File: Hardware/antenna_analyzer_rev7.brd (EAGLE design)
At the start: 99.1 x 78.7 mm, 42 parts, among them J1 DC_JACK, P1 SOLDER_PAD_35_HOLE, P2 SOLDER_PAD_35_HOLE, P3 SOLDER_PAD_35_HOLE, U1 ARDUINO_PRO_MICRO, U2 AD9850_MOD, U3 6002_OP_AMP, U5 SWITCHING_REGULATOR

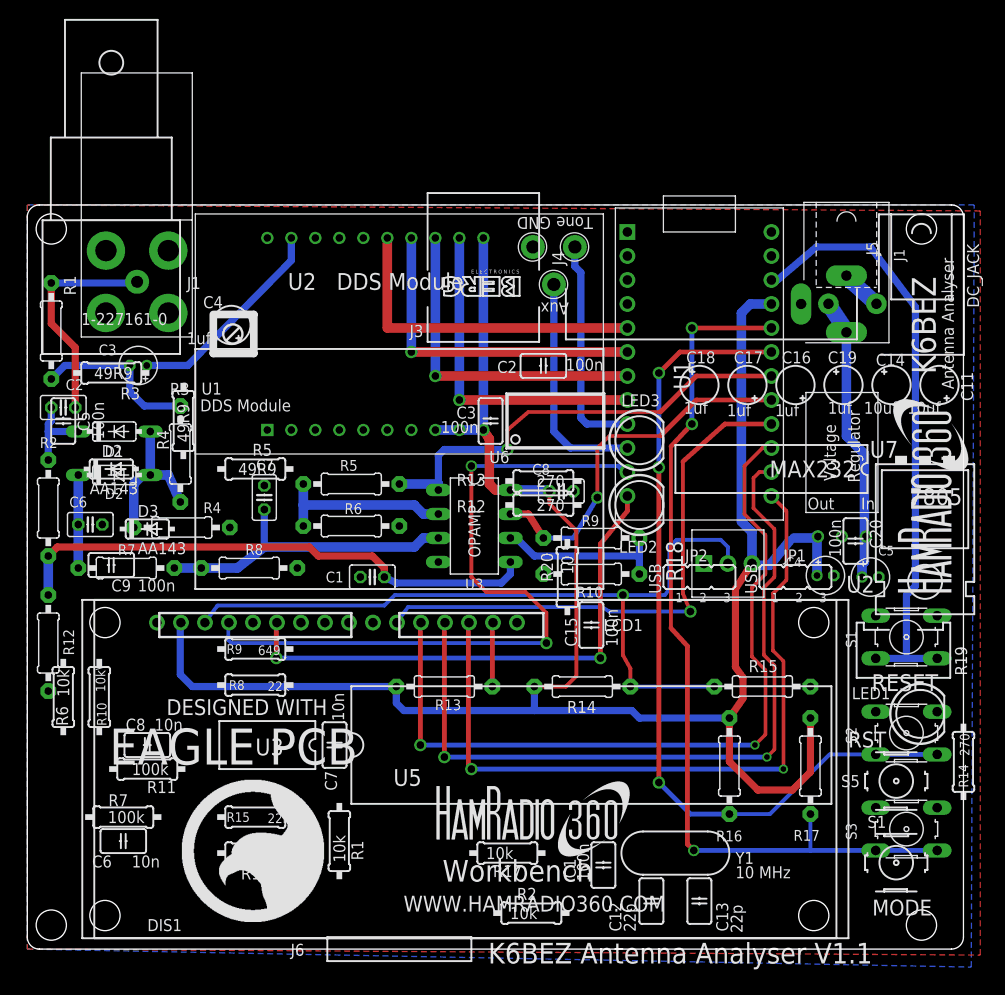
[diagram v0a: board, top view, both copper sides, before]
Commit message: 4X6UB Modifications
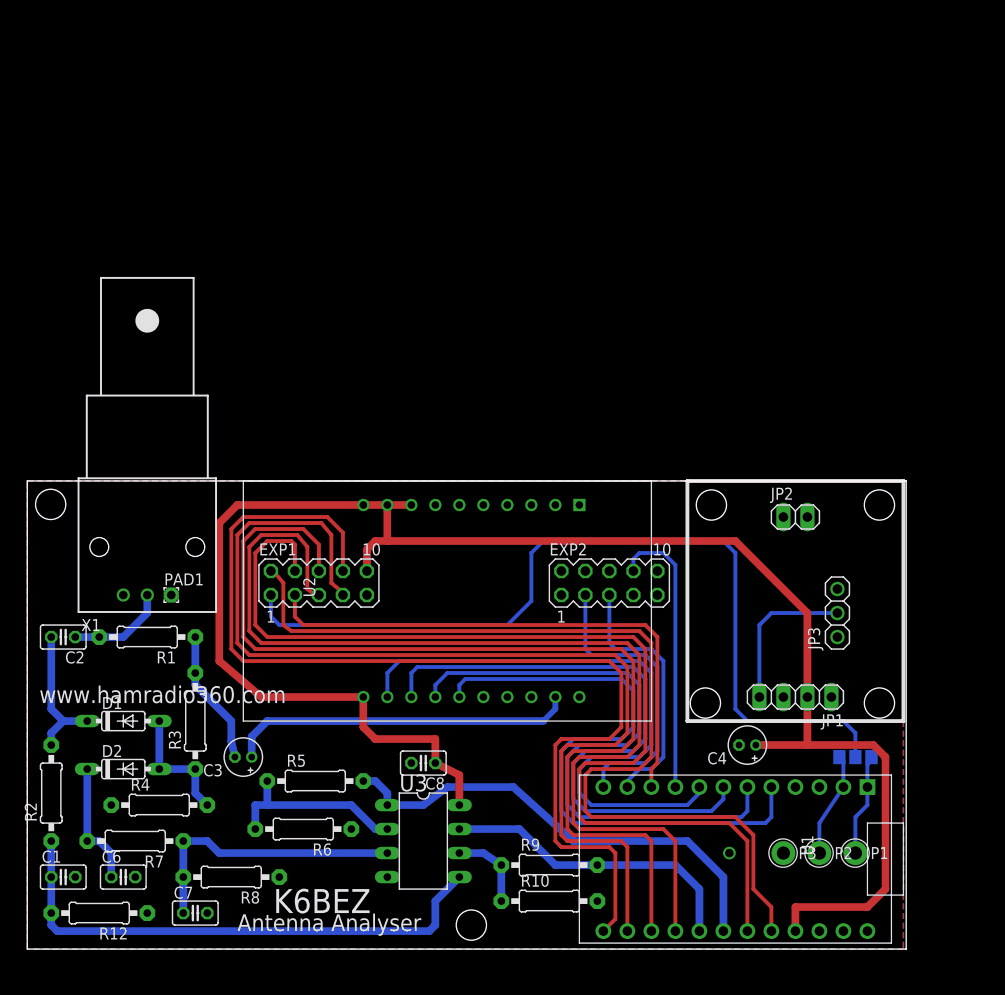
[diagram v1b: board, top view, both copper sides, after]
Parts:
- removed C5: 10uf, resistor:E1,8-4
- removed CON1: (no value), srs_lib_4:BNC-SMALL
- removed J1: DC_JACK, srs_lib_2:DC_COAXIAL_JACK
- removed LCD1: LCD_2_16, srs_lib_4:LCD_2X16
- removed R13: 10, adafruit:0207/10
- removed R14, R16, R17: 10k, adafruit:0207/10
- removed R15: 649, adafruit:0207/10
- removed R18: (no value), Discrete:3362U
- removed S1: RESET, switch-omron:B3F-10XX
- removed S2: MODE, switch-omron:B3F-10XX
- removed S3: BAND, switch-omron:B3F-10XX
- removed U$1, U$2: (no value), Eagle logo:CS-2016-LOGO-15MM
- removed U5: SWITCHING_REGULATOR, srs_new:SWITCHING_REGULATOR
- added EXP1, EXP2: (no value), con-lstb:MA05-2
- added JMP1: 0R-JUMPA, jump-0r-smd:A0R-JMP
- added JP1: (no value), pinhead:1X04
- added JP2: (no value), pinhead:1X02
- added JP3: (no value), adafruit:1X03
- added PAD1: (no value), wirepad:1,6/0,9
- added X1: 1-227161-0, con-coax:AMP_227161
- moved P1 70.7 mm to (87.6, 10.2)
- moved P3 69.4 mm to (80.0, 10.2)
- moved P2 66.4 mm to (83.8, 10.2)
- moved U1 64.0 mm to (88.9, 17.1), turned to 270 degrees
- moved C1 45.6 mm to (3.81, 7.62), turned to 0 degrees
- moved C7 44.6 mm to (17.8, 3.81), turned to 0 degrees
- moved C3 42.9 mm to (22.9, 20.3)
- moved C6 37.5 mm to (10.2, 7.62)
- moved R10 34.9 mm to (55.2, 5.08), turned to 0 degrees
- moved R9 34.9 mm to (55.2, 8.89), turned to 0 degrees
- moved R1 33.9 mm to (12.7, 33.0), turned to 180 degrees
- moved U3 33.8 mm to (41.9, 11.4)
- moved R8 32.8 mm to (21.6, 7.62)
- moved R6 32.5 mm to (29.2, 12.7)
- moved C8 32.3 mm to (41.9, 19.7), turned to 180 degrees
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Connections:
- removed net AUX: P2.1, U1.10
- removed net BAND_SEL: R17.1, S3.3, S3.4, U1.20
- removed net MODE_SEL: R16.1, S2.3, S2.4, U1.19
- removed net N$12: S1.3, S1.4, U1.22
- removed net N$37: LCD1.15, R13.1
- removed net N$40: LCD1.3, R14.1, R15.1, R18.2
- removed net TONE: P1.1, U1.9
- new net BEEPER: EXP1.1, JMP1.2
- new net KILL: EXP2.10
- new net N$8: JMP1.3, P2.1, U1.2
- new net POWER_EN: JP1.4, JP3.2
- new net SD_DETECT: EXP2.7
- new net SD_MISO: EXP2.1
- new net SD_MOSI: EXP2.6
- new net SD_SCLK: EXP2.2
- new net SD_SS: EXP2.4
- new net SW_BTN: EXP1.2, U1.20
- new net SW_E1: EXP2.5, U1.11
- new net SW_E2: EXP2.3, U1.12
- new net SW_RST: EXP2.8, U1.9
- net +5V: now also EXP1.10, JP1.2; no longer LCD1.2, R13.2, R14.2, R16.2, R17.2, R18.3, U5.OUT
- net DGND: now also EXP1.9, EXP2.9, JP1.3, JP3.3, PAD1.1, X1.2; no longer C5.-, CON1.G1, CON1.G2, CON1.G3, CON1.G4, J1.1, LCD1.1, LCD1.10, LCD1.16, LCD1.5, LCD1.7, LCD1.8, LCD1.9, R15.2, R18.1, S1.1, S1.2, S2.1, S2.2, S3.1, U5.GND
- net LCD_D4: now also EXP1.5; no longer LCD1.11
- net LCD_D5: now also EXP1.6; no longer LCD1.12
- net LCD_D6: now also EXP1.7; no longer LCD1.13
- net LCD_D7: now also EXP1.8; no longer LCD1.14
- net LCD_E: now also EXP1.3, U1.10; no longer LCD1.6, U1.12
- net LCD_RS: now also EXP1.4, U1.19; no longer LCD1.4, U1.11
- net N$1: now also JMP1.1, P1.1, U1.1; no longer C5.+, J1.3, U5.IN
- net N$7: now also X1.1; no longer CON1.CENTER
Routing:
- net SW_BTN: track 0.00 -> 99.5 mm
- net BAND_SEL: track 95.1 -> 0.00 mm, vias 3 -> 0
- net BEEPER: track 0.00 -> 91.8 mm
- net MODE_SEL: track 89.6 -> 0.00 mm, vias 3 -> 0
- net N$40: track 82.6 -> 0.00 mm, vias 1 -> 0
- net N$12: track 64.8 -> 0.00 mm
- net LCD_D4: track 58.9 -> 109.1 mm, vias 1 -> 0
- net LCD_RS: track 76.9 -> 109.6 mm, vias 2 -> 0
- net LCD_D7: track 79.3 -> 111.4 mm, vias 2 -> 0
- net SW_E2: track 0.00 -> 31.4 mm
- net +5V: track 214.6 -> 183.5 mm
- net DDS_RESET: track 34.9 -> 65.5 mm
- net DDS_UPDATE: track 34.9 -> 65.1 mm, vias 1 -> 0
- net DDS_DATA: track 34.9 -> 65.1 mm, vias 1 -> 0
- net SW_RST: track 0.00 -> 30.0 mm
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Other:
- board size 99.1 x 78.7 mm -> 93 x 49.5 mm
- board text added: "IR-019"
- board text added: "idoroseman.com"
- board text added: "www.hamradio360.com"
- board text removed: "1"
- board text removed: "1-227161-0"
- board text removed: "10"
- board text removed: "10 MHz"
- board text removed: "100k"
- board text removed: "100n"
- board text removed: "10k"
- board text removed: "10k\"
- board text removed: "10n"
- board text removed: "10uf"
- board text removed: "1uf"
- board text removed: "2"
- board text removed: "22k"
- board text removed: "22p"
- board text removed: "270"
- board text removed: "3"
- board text removed: "49R9"
- board text removed: "649"
- board text removed: "7805"
- board text removed: "AA143"
- board text removed: "Aux"
- board text removed: "C1"
- board text removed: "C11"
- board text removed: "C12"
- board text removed: "C13"
- board text removed: "C14"
- board text removed: "C15"
- board text removed: "C16"
- board text removed: "C17"
- board text removed: "C18"
- board text removed: "C19"
- board text removed: "C2"
- board text removed: "C20"
- board text removed: "C3"
- board text removed: "C4"
- board text removed: "C5"
- board text removed: "C6"
- board text removed: "C7"
- board text removed: "C8"
- board text removed: "C9"
- board text removed: "D2"
- board text removed: "D3"
- board text removed: "DC_JACK"
- board text removed: "DDS Module"
- board text removed: "DESIGNED WITH"
- board text removed: "DIS1"
- board text removed: "E L E C T R O N I C S"
- board text removed: "EAGLE PCB"
- board text removed: "GND"
- board text removed: "In"
- board text removed: "J1"
- board text removed: "J3"
- board text removed: "J4"
- board text removed: "J5"
- board text removed: "J6"
- board text removed: "JP1"
- board text removed: "JP2"
- board text removed: "K6BEZ Antenna Analyser V1.1"
- board text removed: "LED1"
- board text removed: "LED2"
- board text removed: "LED3"
- board text removed: "MAX232"
- board text removed: "MODE"
- board text removed: "OPAMP"
- board text removed: "Out"
- board text removed: "PCB Version 7"
- board text removed: "R1"
- board text removed: "R10"
- board text removed: "R11"
- board text removed: "R12"
- board text removed: "R13"
- board text removed: "R14"
- board text removed: "R15"
- board text removed: "R16"
- board text removed: "R17"
- board text removed: "R19"
- board text removed: "R2"
- board text removed: "R20"
- board text removed: "R3"
- board text removed: "R4"
- board text removed: "R5"
- board text removed: "R6"
- board text removed: "R7"
- board text removed: "R8"
- board text removed: "R9"
- board text removed: "RST"
- board text removed: "Regulator"
- board text removed: "S1"
- board text removed: "S5"
- board text removed: "Tone"
- board text removed: "U1"
- board text removed: "U2"
- board text removed: "U3"
- board text removed: "U5"
- board text removed: "U6"
- board text removed: "U7"
- board text removed: "USB"
- board text removed: "Voltage"
- board text removed: "WWW.HAMRADIO360.COM"
- board text removed: "Workbench"
- board text removed: "Y1"
